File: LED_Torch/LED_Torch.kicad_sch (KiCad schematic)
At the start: 4 parts, among them SW1 SW_DIP_x01

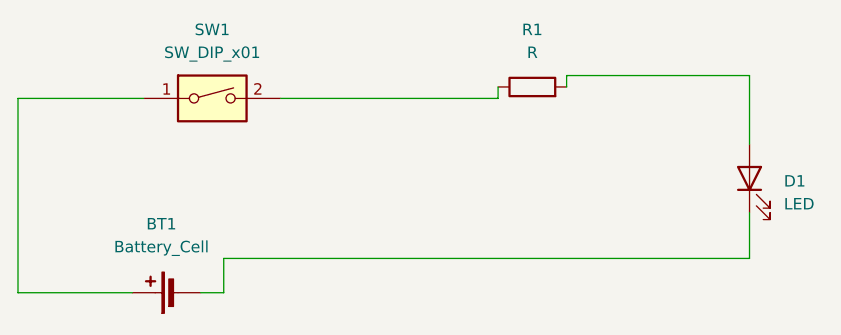
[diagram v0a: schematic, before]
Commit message: IR Sensor
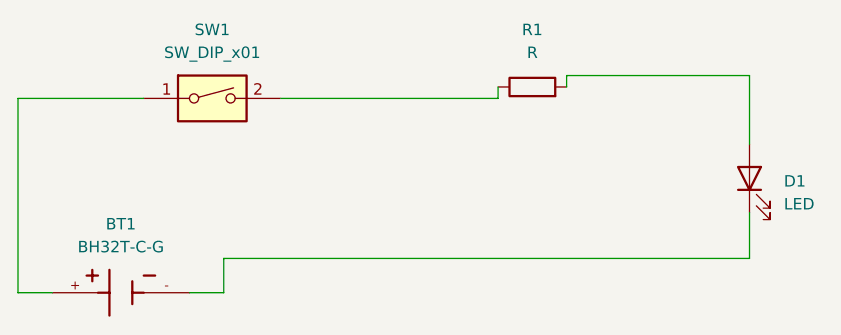
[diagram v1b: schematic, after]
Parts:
- removed BT1: Battery_Cell, Battery:BatteryHolder_Keystone_1058_1x2032, symbol Device:Battery_Cell
- added BT1: BH32T-C-G, New Battery:BAT_BH32T-C-G, symbol New Battery:BH32T-C-G
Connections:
- net at SW1.1: now also BT1.+
- net at D1.1 (K): now also BT1.-
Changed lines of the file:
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@@
-	(wire
-		(pts
-			(xy 115.57 82.55) (xy 128.27 82.55)
-		)
-		(stroke
-			(width 0)
-			(type default)
-		)
-	)
 	(wire
 		(pts
@@
 	(wire
 		(pts
+			(xy 134.62 82.55) (xy 138.43 82.55)
+		)
+		(stroke
+			(width 0)
+			(type default)
+		)
+	)
+	(wire
+		(pts
 			(xy 196.85 73.66) (xy 196.85 78.74)
 		)
@@
 	(wire
 		(pts
+			(xy 115.57 82.55) (xy 119.38 82.55)
+		)
+		(stroke
+			(width 0)
+			(type default)
+		)
+	)
+	(wire
+		(pts
 			(xy 176.53 58.42) (xy 176.53 59.69)
 		)
@@
 		(pts
 			(xy 168.91 60.96) (xy 168.91 59.69)
-		)
-		(stroke
-			(width 0)
-			(type default)
-		)
-	)
-	(wire
-		(pts
-			(xy 138.43 82.55) (xy 135.89 82.55)
 		)
 		(stroke
@@
 	)
 	(symbol
-		(lib_id "Device:Battery_Cell")
-		(at 133.35 82.55 90)
-		(unit 1)
-		(exclude_from_sim no)
-		(in_bom yes)
-		(on_board yes)
-		(dnp no)
-		(fields_autoplaced yes)
-		(property "Reference" "BT1"
-			(at 131.5085 74.93 90)
-			(effects
-				(font
-					(size 1.27 1.27)
-				)
-			)
-		)
-		(property "Value" "Battery_Cell"
-			(at 131.5085 77.47 90)
-			(effects
-				(font
-					(size 1.27 1.27)
-				)
-			)
-		)
-		(property "Footprint" "Battery:BatteryHolder_Keystone_1058_1x2032"
-			(at 131.826 82.55 90)
-			(effects
-				(font
-					(size 1.27 1.27)
-				)
-				(hide yes)
-			)
-		)
-		(property "Datasheet" "~"
-			(at 131.826 82.55 90)
-			(effects
-				(font
-					(size 1.27 1.27)
-				)
-				(hide yes)
-			)
-		)
-		(property "Description" "Single-cell battery"
-			(at 133.35 82.55 0)
-			(effects
-				(font
-					(size 1.27 1.27)
-				)
-				(hide yes)
-			)
-		)
-		(pin "2"
-		)
-		(pin "1"
-		)
-		(instances
-			(project ""
-				(path "/b0e82e06-16d1-4eac-8592-323c27dcfbbd"
-					(reference "BT1")
-					(unit 1)
-				)
-			)
-		)
-	)
-	(symbol
 		(lib_id "Switch:SW_DIP_x01")
 		(at 137.16 60.96 0)
@@
 					(unit 1)
 				)
+			)
+		)
+	)
+	(symbol
+		(lib_id "New Battery:BH32T-C-G")
+		(at 127 82.55 0)
+		(unit 1)
+		(exclude_from_sim no)
+		(in_bom yes)
+		(on_board yes)
+		(dnp no)
+		(fields_autoplaced yes)
+		(property "Reference" "BT1"
+			(at 127 74.93 0)
+			(effects
+				(font
+					(size 1.27 1.27)
+				)
+			)
+		)
+		(property "Value" "BH32T-C-G"
+			(at 127 77.47 0)
+			(effects
+				(font
+					(size 1.27 1.27)
+				)
+			)
+		)
+		(property "Footprint" "New Battery:BAT_BH32T-C-G"
+			(at 127 82.55 0)
+			(effects
+				(font
+					(size 1.27 1.27)
+				)
+				(justify bottom)
+				(hide yes)
+			)
+		)
+		(property "Datasheet" ""
+			(at 127 82.55 0)
+			(effects
+				(font
+					(size 1.27 1.27)
+				)
+				(hide yes)
+			)
+		)
+		(property "Description" ""
+			(at 127 82.55 0)
+			(effects
+				(font
+					(size 1.27 1.27)
+				)
+				(hide yes)
+			)
+		)
+		(property "MF" "MPD"
+			(at 127 82.55 0)
+			(effects
+				(font
+					(size 1.27 1.27)
+				)
+				(justify bottom)
+				(hide yes)
+			)
+		)
+		(property "MAXIMUM_PACKAGE_HEIGHT" "6.80mm"
+			(at 127 82.55 0)
+			(effects
+				(font
+					(size 1.27 1.27)
+				)
+				(justify bottom)
+				(hide yes)
+			)
+		)
+		(property "Package" "None"
+			(at 127 82.55 0)
+			(effects
+				(font
+					(size 1.27 1.27)
+				)
+				(justify bottom)
+				(hide yes)
+			)
+		)
+		(property "Price" "None"
+			(at 127 82.55 0)
+			(effects
+				(font
+					(size 1.27 1.27)
+				)
+				(justify bottom)
+				(hide yes)
+			)
+		)
+		(property "Check_prices" "https://www.snapeda.com/parts/BH32T-C-G/MPD/view-part/?ref=eda"
+			(at 127 82.55 0)
+			(effects
+				(font
+					(size 1.27 1.27)
+				)
+				(justify bottom)
+				(hide yes)
+			)
+		)
+		(property "STANDARD" "Manufacturer Recommendations"
+			(at 127 82.55 0)
+			(effects
+				(font
+					(size 1.27 1.27)
+				)
+				(justify bottom)
+				(hide yes)
+			)
+		)
+		(property "PARTREV" "B"
+			(at 127 82.55 0)
+			(effects
+				(font
+					(size 1.27 1.27)
+				)
+				(justify bottom)
+				(hide yes)
+			)
+		)
+		(property "SnapEDA_Link" "https://www.snapeda.com/parts/BH32T-C-G/MPD/view-part/?ref=snap"
+			(at 127 82.55 0)
+			(effects
+				(font
+					(size 1.27 1.27)
+				)
+				(justify bottom)
+				(hide yes)
+			)
+		)
+		(property "MP" "BH32T-C-G"
+			(at 127 82.55 0)
+			(effects
+				(font
+					(size 1.27 1.27)
+				)
+				(justify bottom)
+				(hide yes)
+			)
+		)
+		(property "Description_1" "\n                        \n                            Battery Holder (Open) Coin, 20.0mm 1 Cell PC Pin\n                        \n"
+			(at 127 82.55 0)
+			(effects
+				(font
+					(size 1.27 1.27)
+				)
+				(justify bottom)
+				(hide yes)
+			)
+		)
+		(property "Availability" "In Stock"
+			(at 127 82.55 0)
+			(effects
+				(font
+					(size 1.27 1.27)
+				)
+				(justify bottom)
+				(hide yes)
+			)
+		)
+		(property "MANUFACTURER" "MPD"
+			(at 127 82.55 0)
+			(effects
+				(font
+					(size 1.27 1.27)
+				)
+				(justify bottom)
+				(hide yes)
+			)
+		)
+		(pin "+"
+		)
+		(pin "-"
+		)
+		(instances
+			(project ""
+				(path "/b0e82e06-16d1-4eac-8592-323c27dcfbbd"
+					(reference "BT1")
+					(unit 1)
+				)
